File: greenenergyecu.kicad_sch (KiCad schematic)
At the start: 35 parts, among them J22 USB_B_Mini, M1 Module-power_12and5V-0.3, M2 Module-knock-0.2, M3 Module-vr-discrete-0.5, M4 Module-vr-max9924-0.1, M5 Module-wbo-0.5, M6 Module:mega-mcu100/0.3, M7 Module-can-0.1, M8 Module-motor-driver-0.1, P1 368255-2, Q1 AO3400A, U1 BTS6143D

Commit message: wew
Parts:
- P1: LCSC (none) -> C392284
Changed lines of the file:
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@@
+			)
+		)
+		(property "LCSC" "C392284"
+			(at 27.94 180.34 0)
+			(effects
+				(font
+					(size 1.27 1.27)
+				)
+				(hide yes)
 			)
 		)
@@
 			(at 27.94 356.87 0)
 			(effects
+				(font
+					(size 1.27 1.27)
+				)
+				(hide yes)
+			)
+		)
+		(property "LCSC" "C392284"
+			(at 27.94 356.87 0)
+			(effects

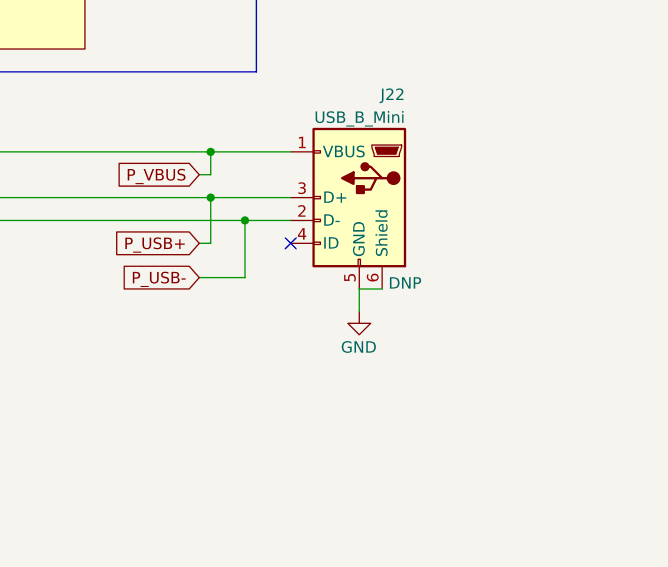
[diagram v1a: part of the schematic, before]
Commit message: ww
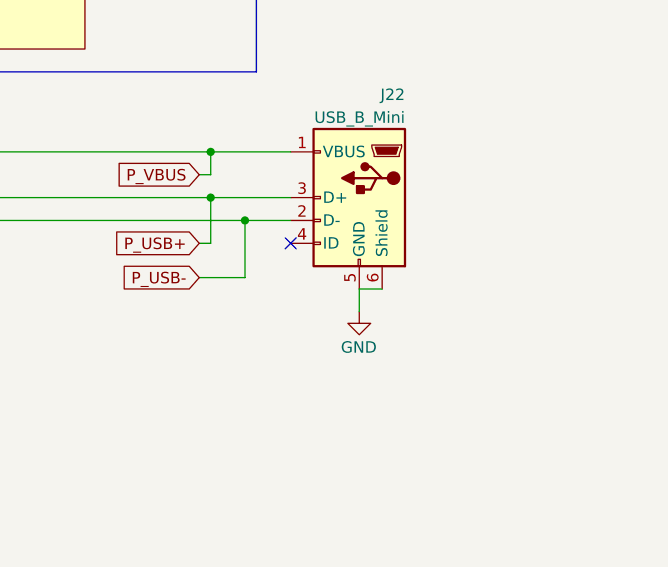
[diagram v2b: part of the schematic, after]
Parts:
- J22: LCSC (none) -> C2682228; MyComment DNP -> (none)
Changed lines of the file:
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@@
 			)
 		)
-		(property "LCSC" ""
+		(property "LCSC" "C2682228"
 			(at 394.97 302.26 0)
 			(effects
@@
 			)
 		)
-		(property "MyComment" "DNP"
+		(property "MyComment" ""
 			(at 400.05 311.785 0)
 			(effects

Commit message: ww
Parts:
- D1: LCSC (none) -> C5119706
- Q1: LCSC (none) -> C20917
- U1: LCSC (none) -> C95232
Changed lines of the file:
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@@
 			)
 		)
+		(property "LCSC" "C5119706"
+			(at 414.02 194.31 0)
+			(effects
+				(font
+					(size 1.27 1.27)
+				)
+				(hide yes)
+			)
+		)
 		(pin "2"
 		)
@@
 			)
 		)
+		(property "LCSC" "C20917"
+			(at 405.13 227.33 0)
+			(effects
+				(font
+					(size 1.27 1.27)
+				)
+				(hide yes)
+			)
+		)
 		(pin "2"
 		)
@@
 			(effects
 				(font
+					(size 1.27 1.27)
+				)
+				(hide yes)
+			)
+		)
+		(property "LCSC" "C95232"
+			(at 410.21 209.55 90)
+			(effects
+				(font

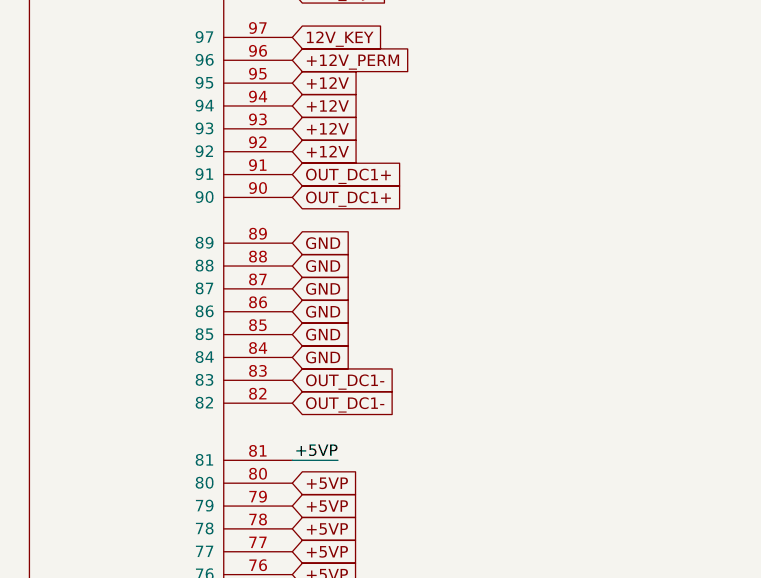
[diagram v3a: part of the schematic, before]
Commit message: w
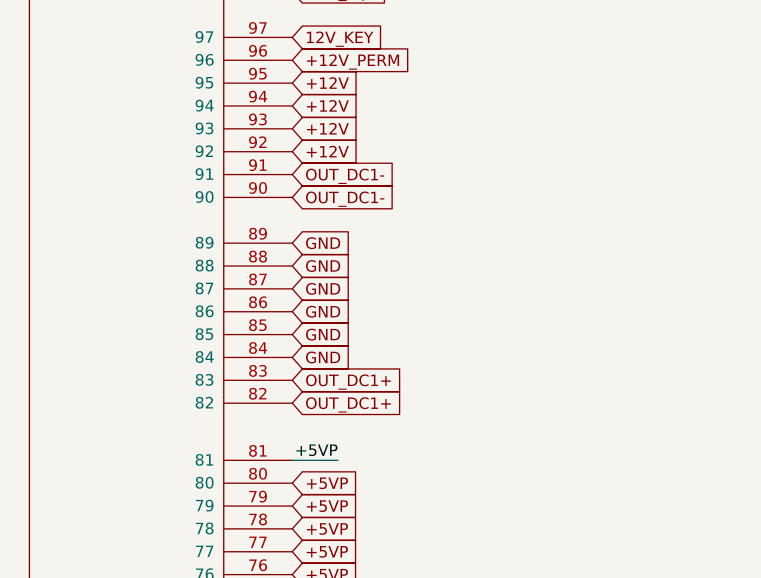
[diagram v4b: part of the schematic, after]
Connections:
- net OUT_DC1+: now also P1.82, P1.83; no longer P1.90, P1.91
- net OUT_DC1-: now also P1.90, P1.91; no longer P1.82, P1.83
